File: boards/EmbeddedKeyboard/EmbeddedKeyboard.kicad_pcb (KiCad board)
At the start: 2 copper layers, 64.5 x 33 mm, 41 parts, among them J1 S2B-PH-SM4-TB, J2 Conn_01x20_Pin, J8 USB_C_Receptacle_USB2.0_14P, Q1 DMN3135LVT-7, SW1 SLIDE SWITCH, U1 LM3671MFX-3.3_NOPB, U2 MCP73831T-2ACI_OT, U3 ESP32-WROOM-32E, U5 CH340C

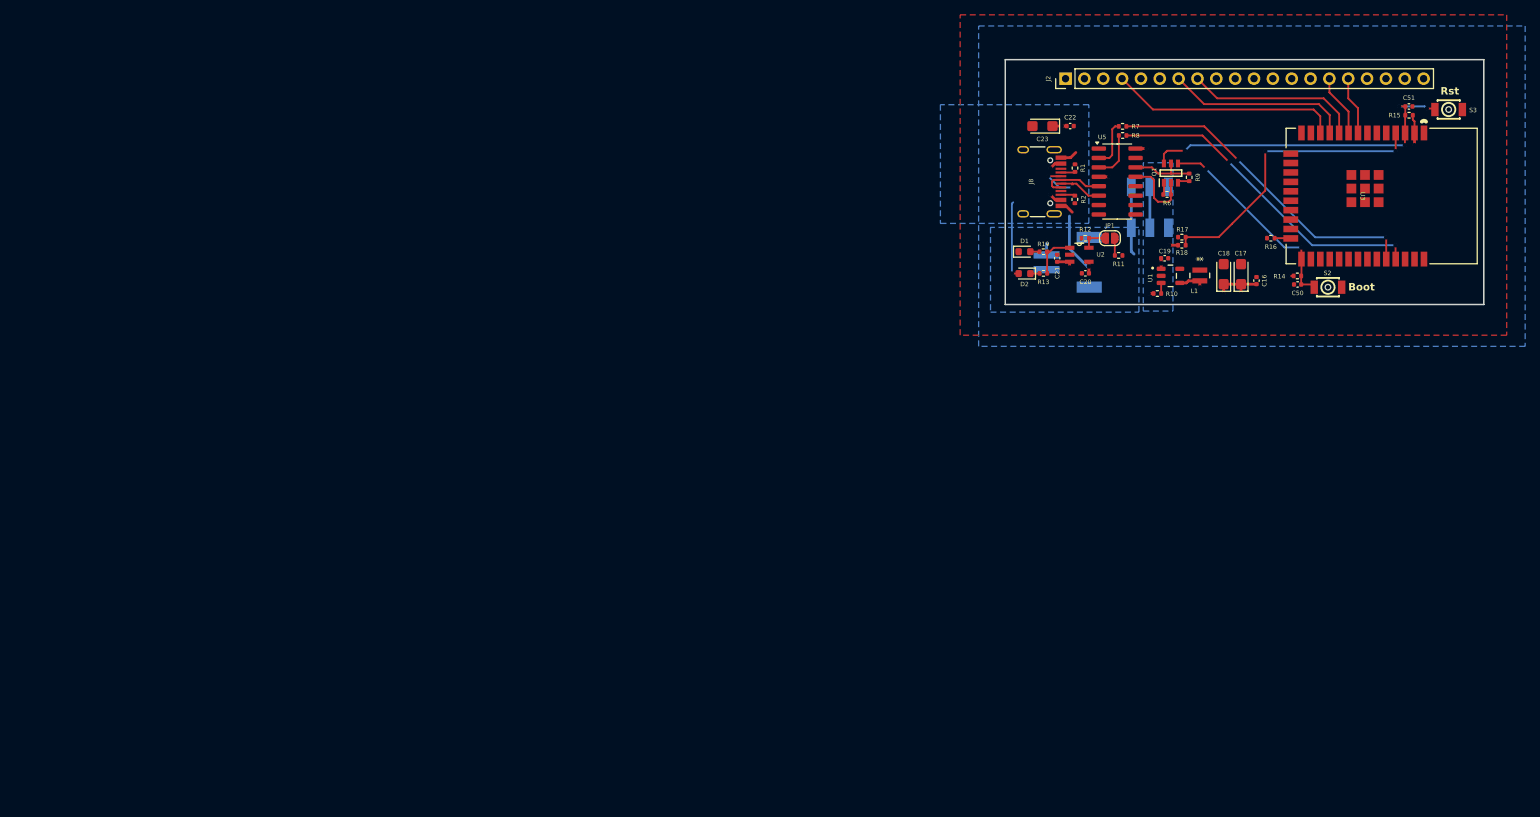
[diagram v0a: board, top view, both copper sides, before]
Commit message: Enough spec to communicate intent
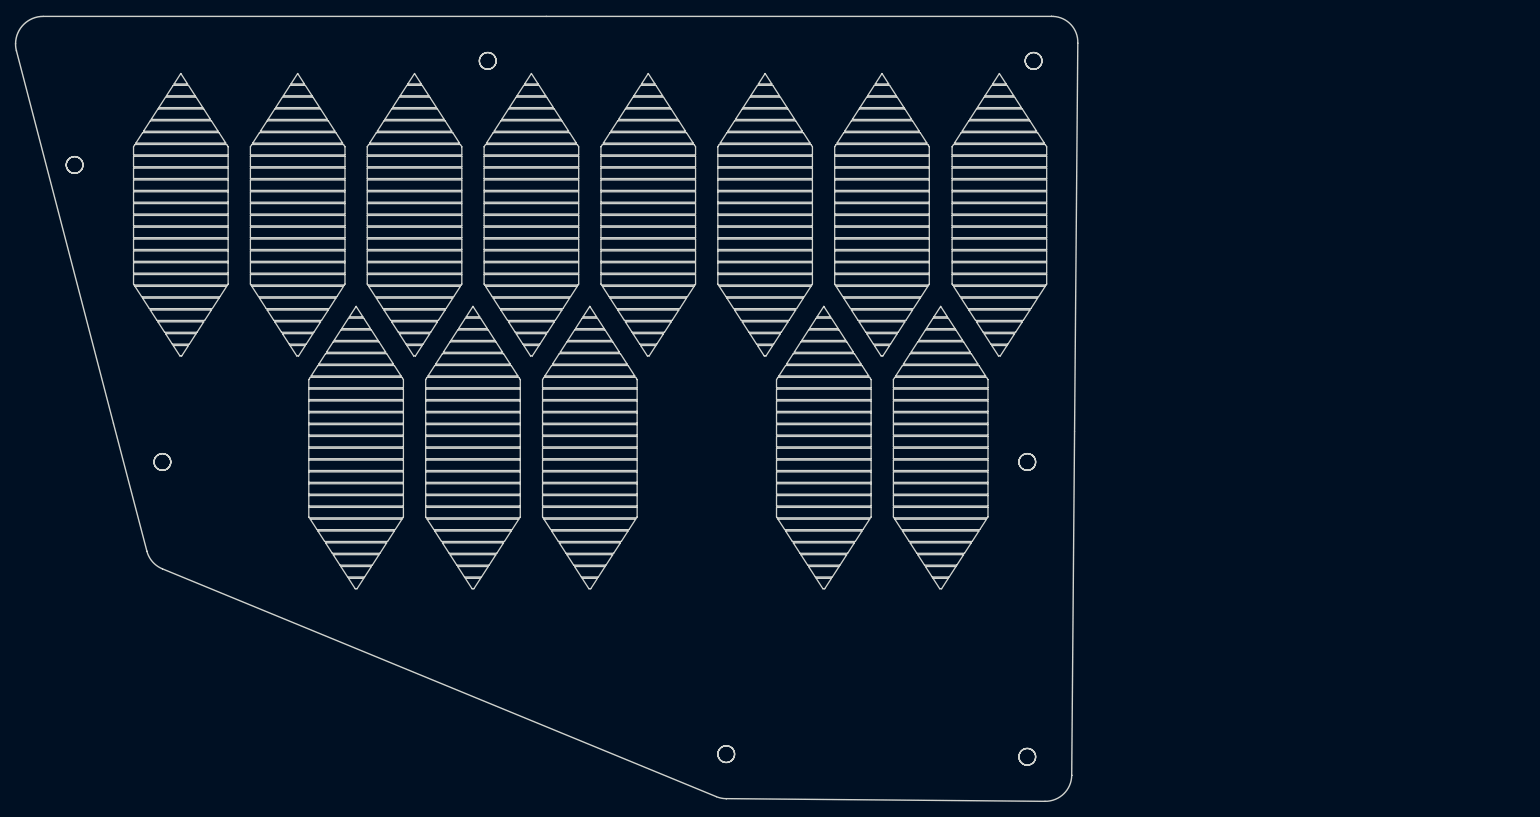
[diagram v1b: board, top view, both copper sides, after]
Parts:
- removed C16, C22, C50, C51: 100nF, Capacitor_SMD:C_0402_1005Metric
- removed C17, C18, C23: 10uF, Capacitor_Tantalum_SMD:CP_EIA-3216-10_Kemet-I
- removed C19, C20, C21: 10uF, Capacitor_SMD:C_0402_1005Metric
- removed D1: GREEN LED (DONE), LED_SMD:LED_0603_1608Metric
- removed D2: RED LED (CHARGING), LED_SMD:LED_0603_1608Metric
- removed J1: S2B-PH-SM4-TB, S2B-PH-SM4-TB:S2B-PH-SM4-TB
- removed J2: Conn_01x20_Pin, Connector_PinHeader_2.54mm:PinHeader_1x20_P2.54mm_Vertical
- removed J8: USB_C_Receptacle_USB2.0_14P, marbastlib-various.pretty:USB_C_Receptacle_HRO_TYPE-C-31-M-12
- removed JP1: SolderJumper, Jumper:SolderJumper-2_P1.3mm_Open_RoundedPad1.0x1.5mm
- removed L1: 2.2uH, NRH2412T2R2MNGH:NRH2412T2R2MNGH
- removed Q1: DMN3135LVT-7, symbols:SOT95P280X100-6N
- removed R1, R2: 5.1k, Resistor_SMD:R_0402_1005Metric
- removed R10: 100K, Resistor_SMD:R_0402_1005Metric
- removed R11: 2.5K, Resistor_SMD:R_0402_1005Metric
- removed R12, R14, R15, R16, R6, R7, R8, R9: 10K, Resistor_SMD:R_0402_1005Metric
- removed R13, R19: 1K, Resistor_SMD:R_0402_1005Metric
- removed R17, R18: 51K, Resistor_SMD:R_0402_1005Metric
- removed S2, S3: TS-1064S-A1B2-D4, TS-1064S-A1B2-D4:KEY-SMD_L3.0-W2.5-LS4.0
- removed SW1: SLIDE SWITCH, JS202011SCQN:JS202011SCQN
- removed U1: LM3671MFX-3.3_NOPB, LM3671MFX-3.3_NOPB:LM3671MFX-3.3_NOPB
- removed U2: MCP73831T-2ACI_OT, MCP73831T-2ACI-OT:MCP73831T-2ACI-OT
- removed U3: ESP32-WROOM-32E, ESP32-WROOM-32E:ESP32-WROOM-32E
- removed U5: CH340C, Package_SO:SOIC-16_3.9x9.9mm_P1.27mm
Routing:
- net /Rst: track 45.4 -> 0.00 mm, vias 4 -> 0
- net /UTx: track 44.3 -> 0.00 mm, vias 2 -> 0
- net /URx: track 44.2 -> 0.00 mm, vias 2 -> 0
- net /Bat: track 39.8 -> 0.00 mm, vias 2 -> 0
- net /DC: track 31.1 -> 0.00 mm
- net /G0: track 28.2 -> 0.00 mm, vias 2 -> 0
- net +5V: track 25.5 -> 0.00 mm, vias 5 -> 0
- net /SCK: track 24.8 -> 0.00 mm
- net /MOSI: track 23.6 -> 0.00 mm
- net +3.3V: track 18.6 -> 0.00 mm, vias 7 -> 0
- net /D-: track 12.0 -> 0.00 mm, vias 2 -> 0
- net VB+: track 11.7 -> 0.00 mm, vias 1 -> 0
- net /DTR: track 9.97 -> 0.00 mm
- net /RTS: track 8.94 -> 0.00 mm
- net VBo+: track 8.85 -> 0.00 mm, vias 3 -> 0
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- removed copper zone on B.Cu, net +3.3V
- removed copper zone on B.Cu, net +5V
- removed copper zone on F.Cu, net GND
- removed copper zone on B.Cu, net VB+
- removed copper zone on B.Cu, net VBo+
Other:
- board size 64.5 x 33 mm -> 143.2 x 105.8 mm
- board text removed: "Boot"
- board text removed: "Rst"
